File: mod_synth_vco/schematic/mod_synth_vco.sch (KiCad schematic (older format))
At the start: 15 parts

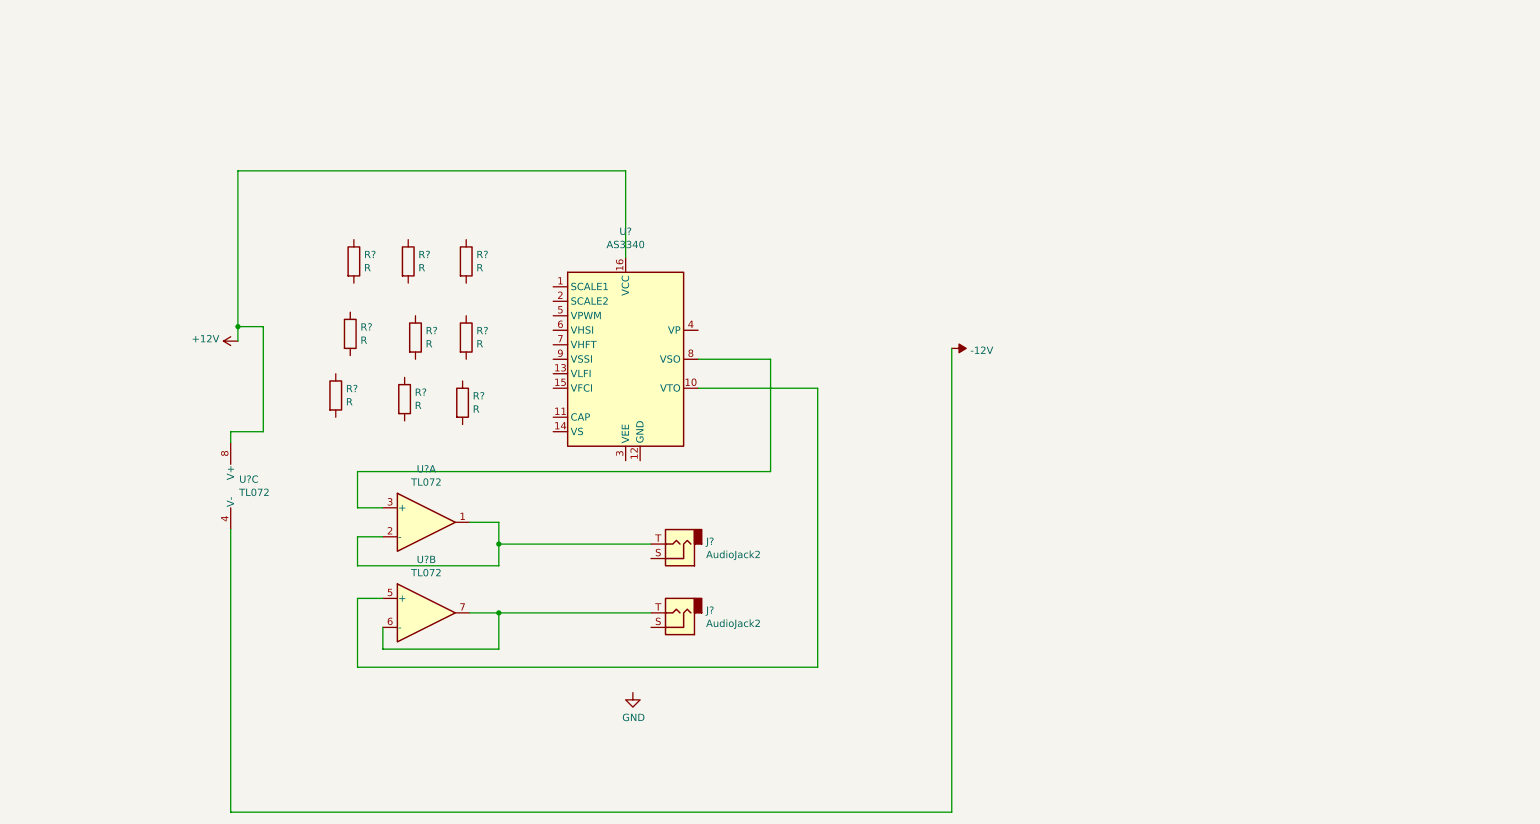
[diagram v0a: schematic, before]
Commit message: Update schematic for vco
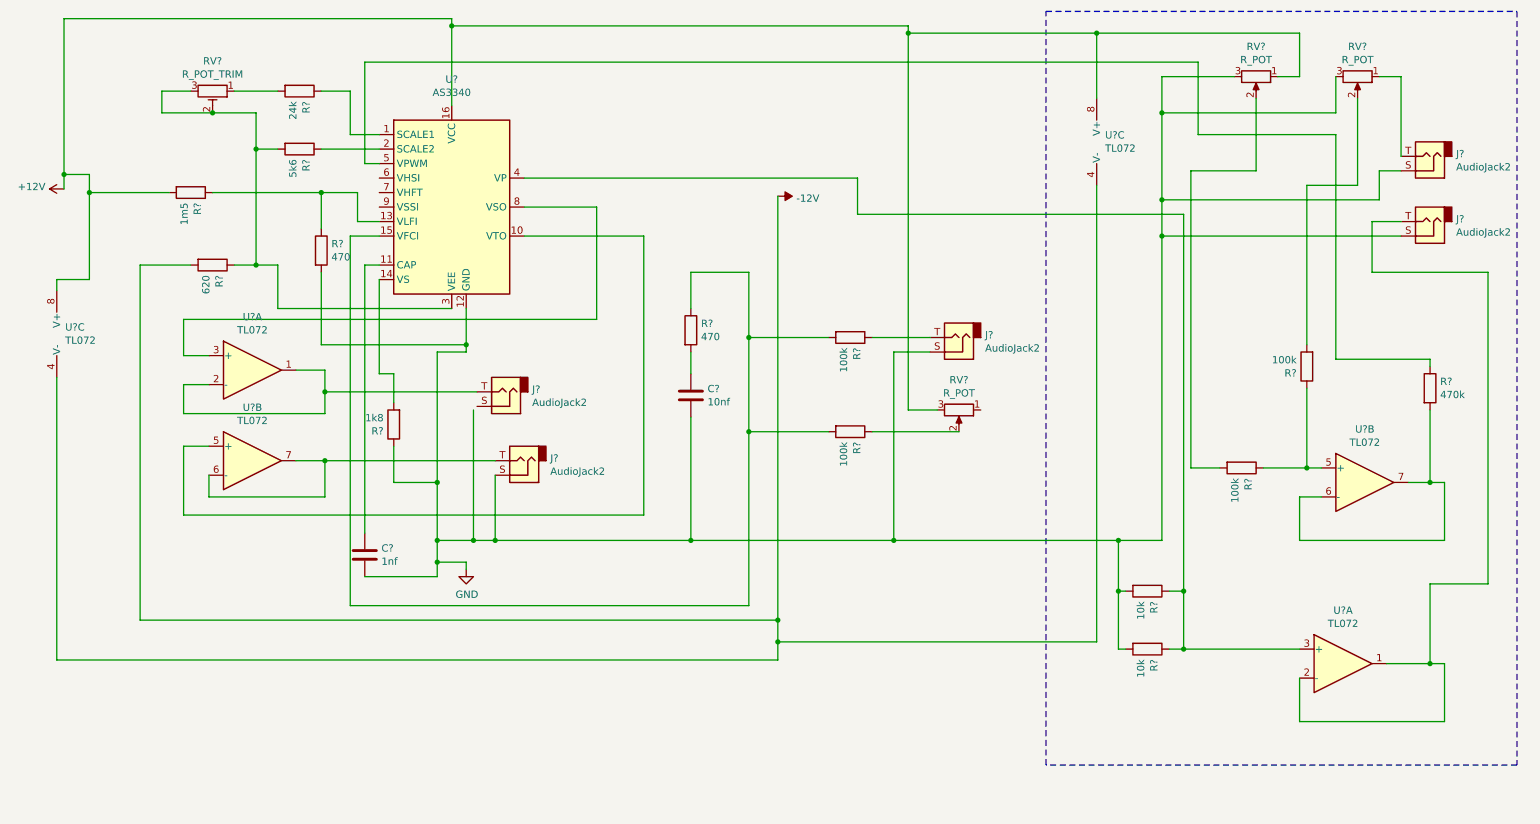
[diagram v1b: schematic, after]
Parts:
- added C?: 10nf, symbol Device:C
- added C?: 1nf, symbol Device:C
- added J? (x3): AudioJack2, symbol Connector:AudioJack2
- added R? (x2): 100k, symbol Device:R
- added R? (x2): 10k, symbol Device:R
- added R?: 470k, symbol Device:R
- added RV? (x3): R_POT, symbol Device:R_POT
- added RV?: R_POT_TRIM, symbol Device:R_POT_TRIM
- added U? (x3): TL072, symbol Amplifier_Operational:TL072
- R?: value R -> 24k
- R?: value R -> 1m5
- R?: value R -> 5k6
- R? (x2): value R -> 100k
- R?: value R -> 620
- R?: value R -> 1k8
- R? (x2): value R -> 470
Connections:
- net +12V: now also R?.2, RV?.1, RV?.3, U?.8 (V+)
- net -12V: now also R?.2, U?.4 (V-)
- net GND: now also J?.S, R?.1, R?.2, U?.12 (GND), C?.2, C?.2, J?.S, J?.S, J?.S, R?.2, R?.2, RV?.3, RV?.3
- net at U?.1 (SCALE1): now also R?.1
- net at U?.11 (CAP): now also C?.1
- net at U?.13 (VLFI): now also R?.1, R?.1
- net at U?.14 (VS): now also R?.2
- net at U?.15 (VFCI): now also R?.1, R?.2, R?.2
- net at U?.2 (SCALE2): now also R?.1
- net at U?.3 (VEE): now also R?.1, R?.2, RV?.2, RV?.3
- net at U?.4 (VP): now also R?.1, R?.1, U?.3 (+)
- net at U?.5 (VPWM): now also R?.1
- net at R?.2: now also RV?.1
- net at R?.1: now also J?.T
- net at R?.2: now also C?.1
- net at R?.1: now also RV?.2
- new net: J?.T, RV?.1
- new net: R?.2, RV?.2 (x2)
- new net: J?.T, U?.1, U?.2 (-)
- new net: R?.1, R?.1, U?.5 (+)
- new net: R?.2, U?.6 (-), U?.7
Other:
- moved on the sheet: J?, R?, U?, U?A, U?B, U?C
